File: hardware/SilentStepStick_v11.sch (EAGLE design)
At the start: 30 parts, among them IC1 TMC2100_QFN36, X1 PASSER-07, X2 PASSER-07

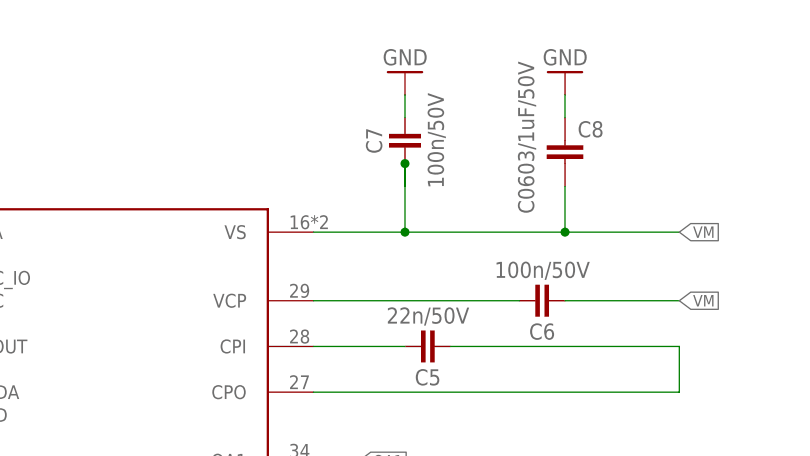
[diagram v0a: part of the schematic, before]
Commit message: updated layout and schematics
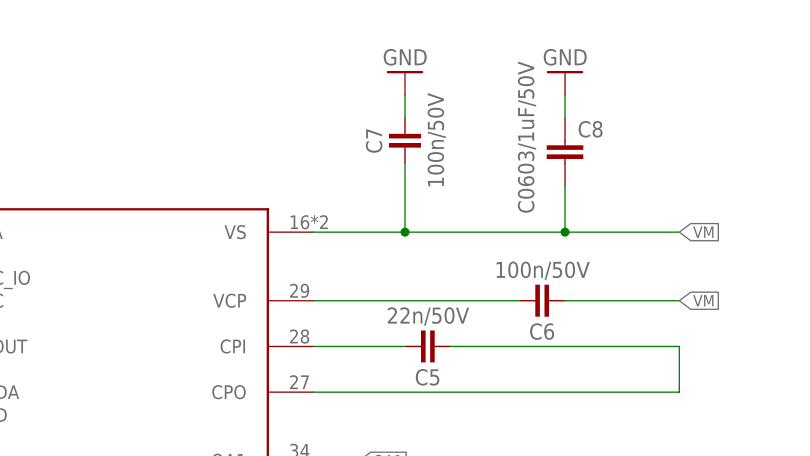
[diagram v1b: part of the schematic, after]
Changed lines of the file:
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@@
 <?xml version="1.0" encoding="utf-8"?>
 <!DOCTYPE eagle SYSTEM "eagle.dtd">
-<eagle version="7.2.0">
+<eagle version="7.5.0">
 <drawing>
 <settings>
@@
 <junction x="168.91" y="149.86"/>
 <pinref part="C7" gate="C" pin="1"/>
-<junction x="151.13" y="157.48"/>
-<wire x1="151.13" y1="157.48" x2="151.13" y2="154.94" width="0.1524" layer="91"/>
-</segment>
-<segment>
+</segment>
+<segment>
